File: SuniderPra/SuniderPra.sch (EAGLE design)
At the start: 16 parts, among them Q1 2SK4017(Q), Q2 2SK4017(Q), U1 GY-521MPU6050, X1 B2P-VH, X2 B2P-VH, X3 B2P-VH

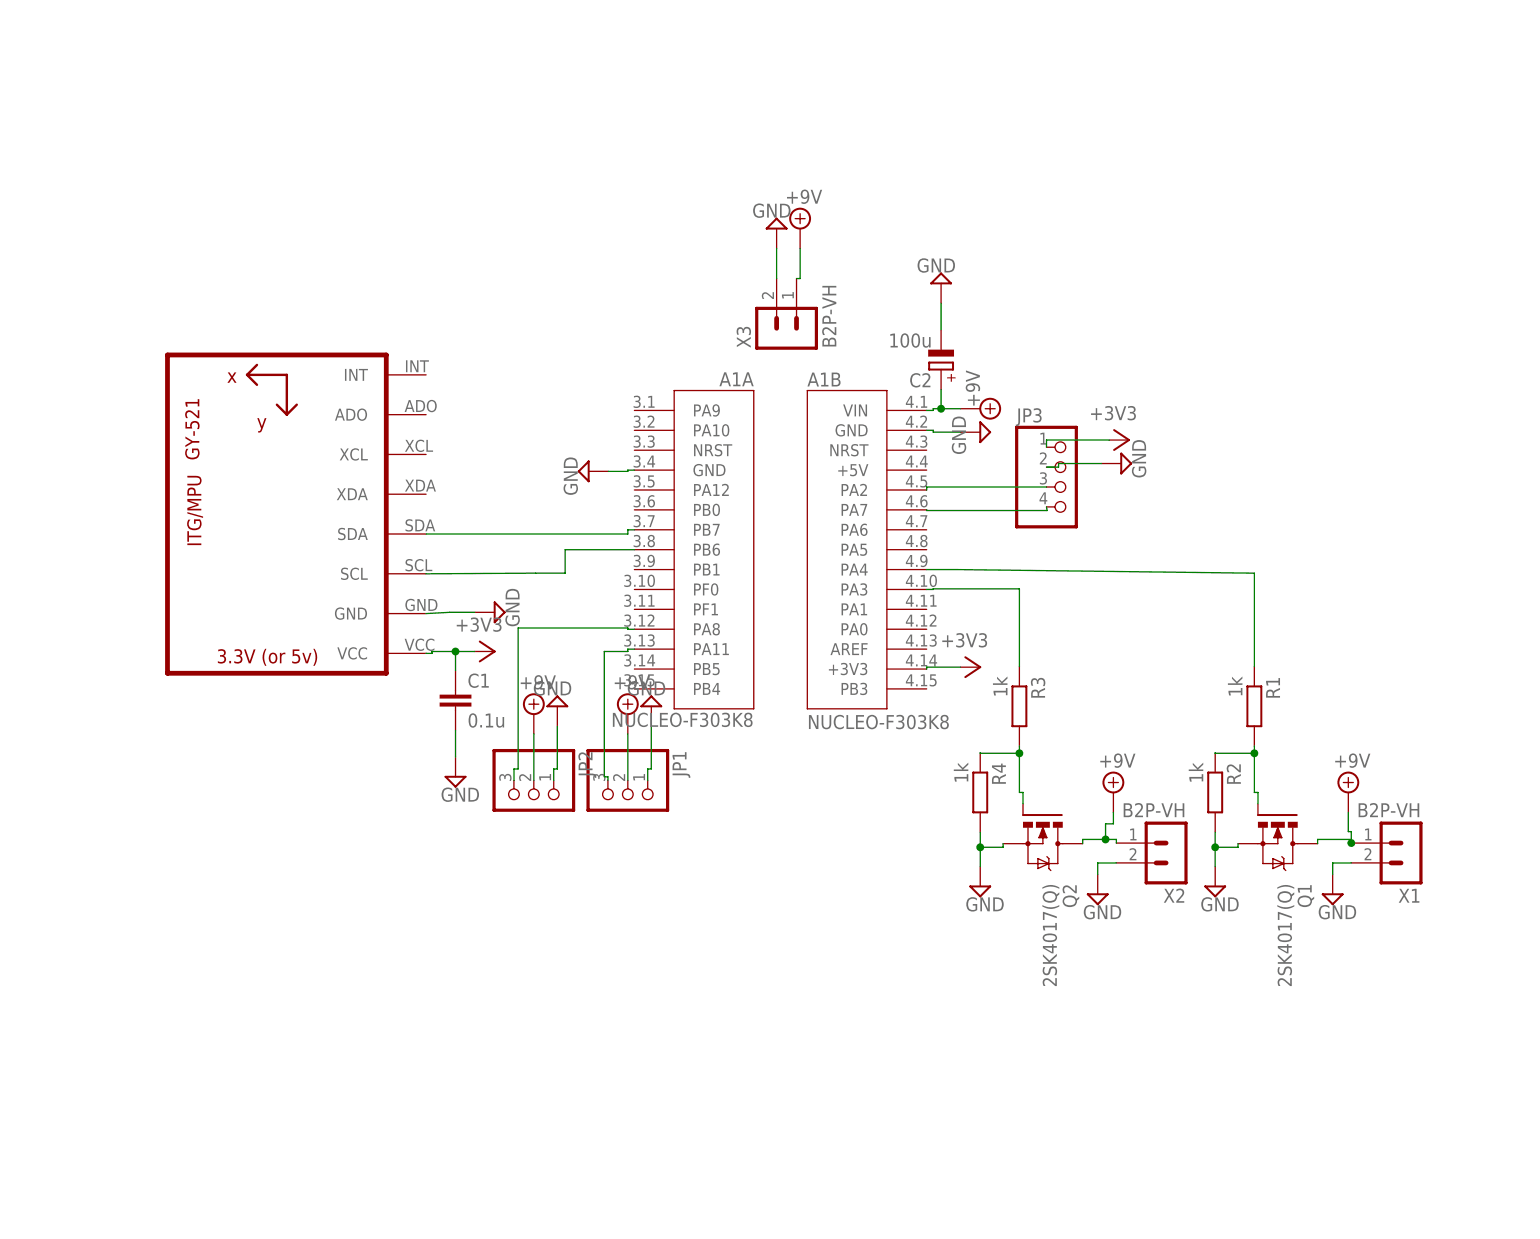
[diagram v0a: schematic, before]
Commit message: Add files via upload
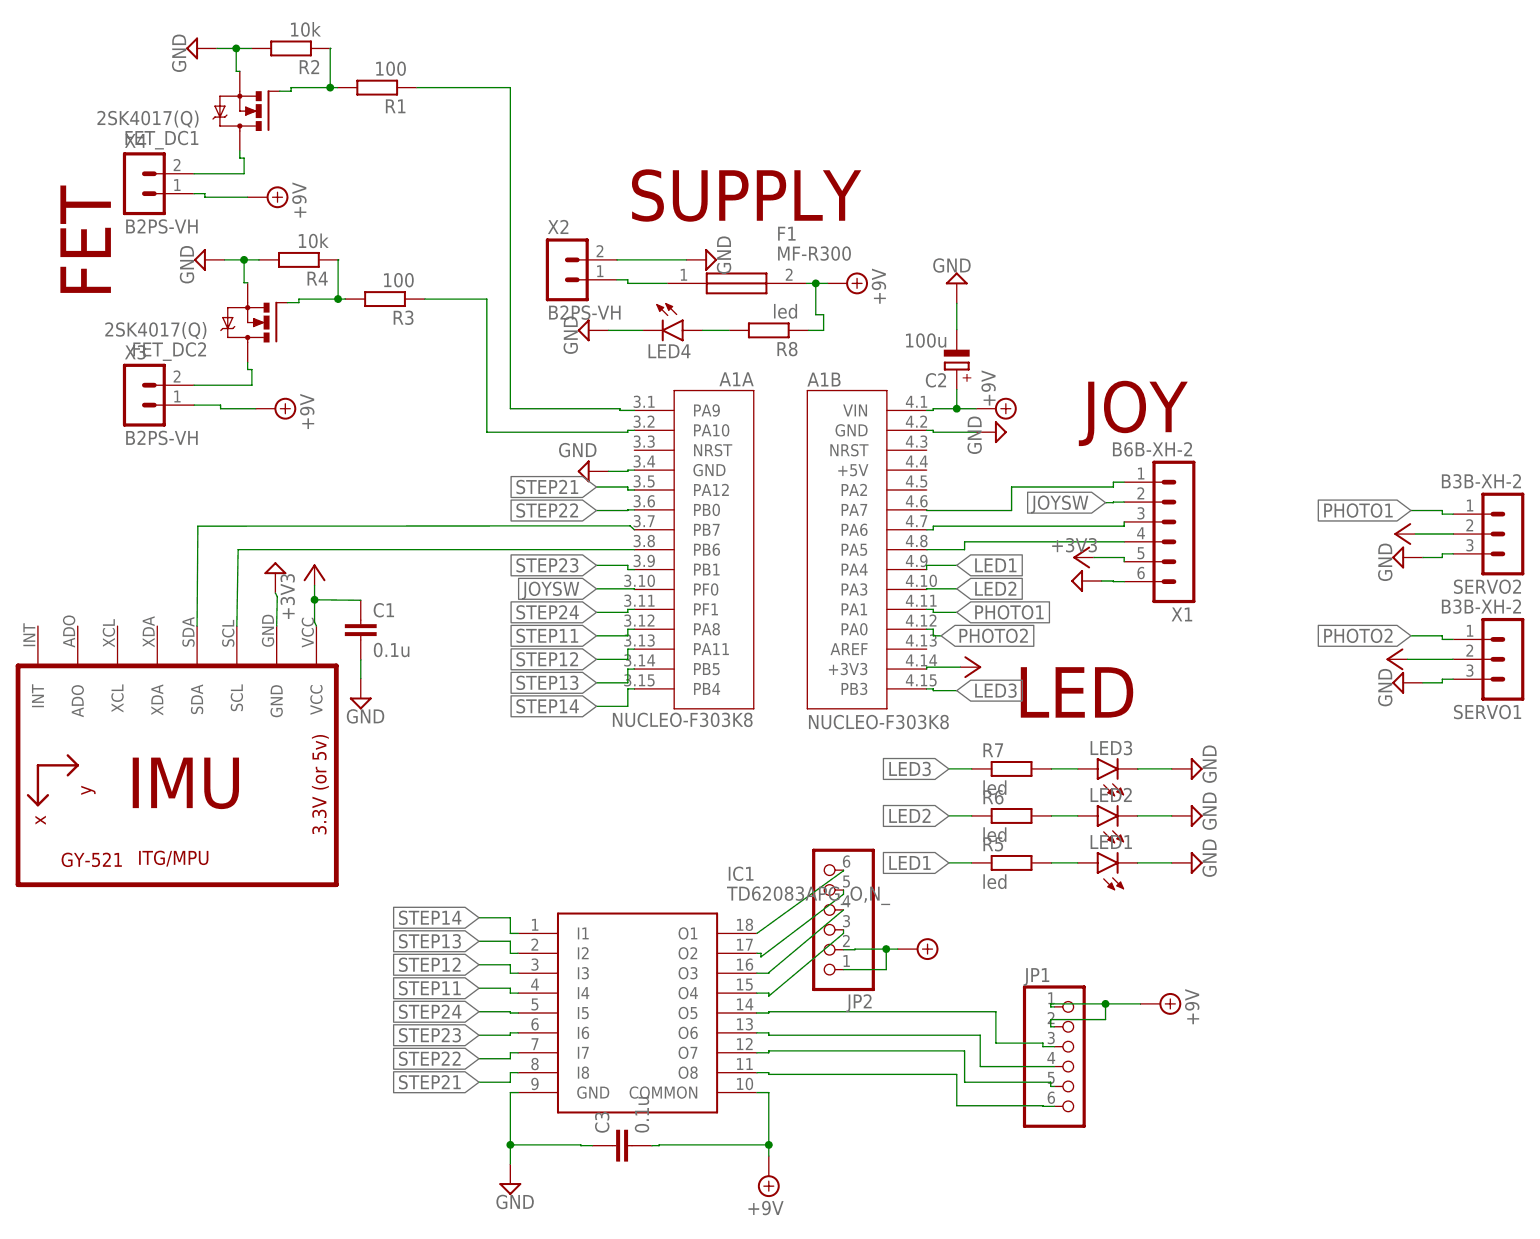
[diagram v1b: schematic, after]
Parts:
- removed JP3: (no value), pinhead:PINHD-1X4
- removed Q1, Q2: 2SK4017(Q), 2SK4017_Q_:2SK4017(Q)
- removed U1: GY-521MPU6050, MPU6050:GY-521MPU6050
- added C3: 0.1u, rcl:C-EU050-024X044
- added F1: MF-R300, MF-R300:MF-R300
- added FET_DC1, FET_DC2: 2SK4017(Q), 2SK4017_Q_:2SK4017(Q)
- added IC1: TD62083APG_O,N_, SamacSys_Parts:TD62083APG_O,N_
- added IMU: GY-521MPU6050, MPU6050:GY-521MPU6050
- added LED1, LED2, LED3, LED4: (no value), led:LED3MM
- added R5, R6, R7, R8: led, rcl:R-EU_0207/7
- added SERVO1, SERVO2: B3B-XH-2, con-JST XH:B3B-XH-2
- added X4: B2PS-VH, con-JST VH:B2PS-VH
- JP1, JP2: device pinhead:PINHD-1X3 -> pinhead:PINHD-1X6
- R1, R3: value 1k -> 100
- R2, R4: value 1k -> 10k
- X1: value B2P-VH -> B6B-XH-2; device con-JST VH:B2P-VH -> con-JST XH:B6B-XH-2
- X2, X3: value B2P-VH -> B2PS-VH; device con-JST VH:B2P-VH -> con-JST VH:B2PS-VH
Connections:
- new net JOYSW: A1A.PF0, X1.2
- new net LED1: A1B.PA4, R5.1
- new net LED2: A1B.PA3, R6.1
- new net LED3: A1B.PB3, R7.1
- new net N$10: FET_DC1.D, X4.2
- new net N$12: IC1.O6, JP1.4
- new net N$13: A1A.PA9, R1.1
- new net N$14: LED1.A, R5.2
- new net N$15: LED3.A, R7.2
- new net N$16: IC1.O5, JP1.3
- new net N$17: IC1.O4, JP2.3
- new net N$18: A1B.PA7, X1.1
- new net N$19: F1.1, X2.1
- new net N$20: A1B.PA6, X1.3
- new net N$21: LED4.A, R8.2
- new net N$22: IC1.O3, JP2.4
- new net N$23: IC1.O2, JP2.5
- new net N$24: IC1.O1, JP2.6
- new net PHOTO1: A1B.PA1, SERVO2.1
- new net PHOTO2: A1B.PA0, SERVO1.1
- new net STEP11: A1A.PA8, IC1.I4
- new net STEP12: A1A.PA11, IC1.I3
- new net STEP13: A1A.PB5, IC1.I2
- new net STEP14: A1A.PB4, IC1.I1
- new net STEP21: A1A.PA12, IC1.I8
- new net STEP22: A1A.PB0, IC1.I7
- new net STEP23: A1A.PB1, IC1.I6
- new net STEP24: A1A.PF1, IC1.I5
- net +3V3: now also IMU.VCC, SERVO1.2, SERVO2.2, X1.5; no longer JP3.1, U1.VCC
- net +9V: now also C3.2, F1.2, IC1.COMMON, JP1.1, JP2.1, R8.1, X4.1; no longer Q1.D, Q2.D, X1.1, X2.1
- net GND: now also C3.1, FET_DC1.S, FET_DC2.S, IC1.GND, IMU.GND, LED1.C, LED2.C, LED3.C, LED4.C, SERVO1.3, SERVO2.3, X1.6; no longer JP1.1, JP2.1, JP3.2, Q1.S, Q2.S, U1.GND, X1.2, X3.2
- net N$1: now also IMU.SCL; no longer U1.SCL
- net N$11: now also LED2.A, R6.2; no longer A1B.PA3, R3.1
- net N$2: now also IMU.SDA; no longer U1.SDA
- net N$3: now also IC1.O8, JP1.6; no longer A1A.PA11, JP1.3
- net N$4: now also IC1.O7, JP1.5; no longer A1A.PA8, JP2.3
- net N$5: now also A1B.PA5, X1.4; no longer A1B.PA4, R1.1
- net N$6: now also FET_DC1.G; no longer Q1.G
- net N$7: now also FET_DC2.D, X3.2; no longer A1B.PA7, JP3.4
- net N$8: now also A1A.PA10, R3.1; no longer A1B.PA2, JP3.3
- net N$9: now also FET_DC2.G; no longer Q2.G
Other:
- note added: "FET"
- note added: "IMU"
- note added: "JOY"
- note added: "LED"
- note added: "SUPPLY"
- moved on the sheet: C1, C2, R1, R2, R3, R4, X2, X3
